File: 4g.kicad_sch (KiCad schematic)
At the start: 1 part, among them J6 Bus_M.2_Socket_B

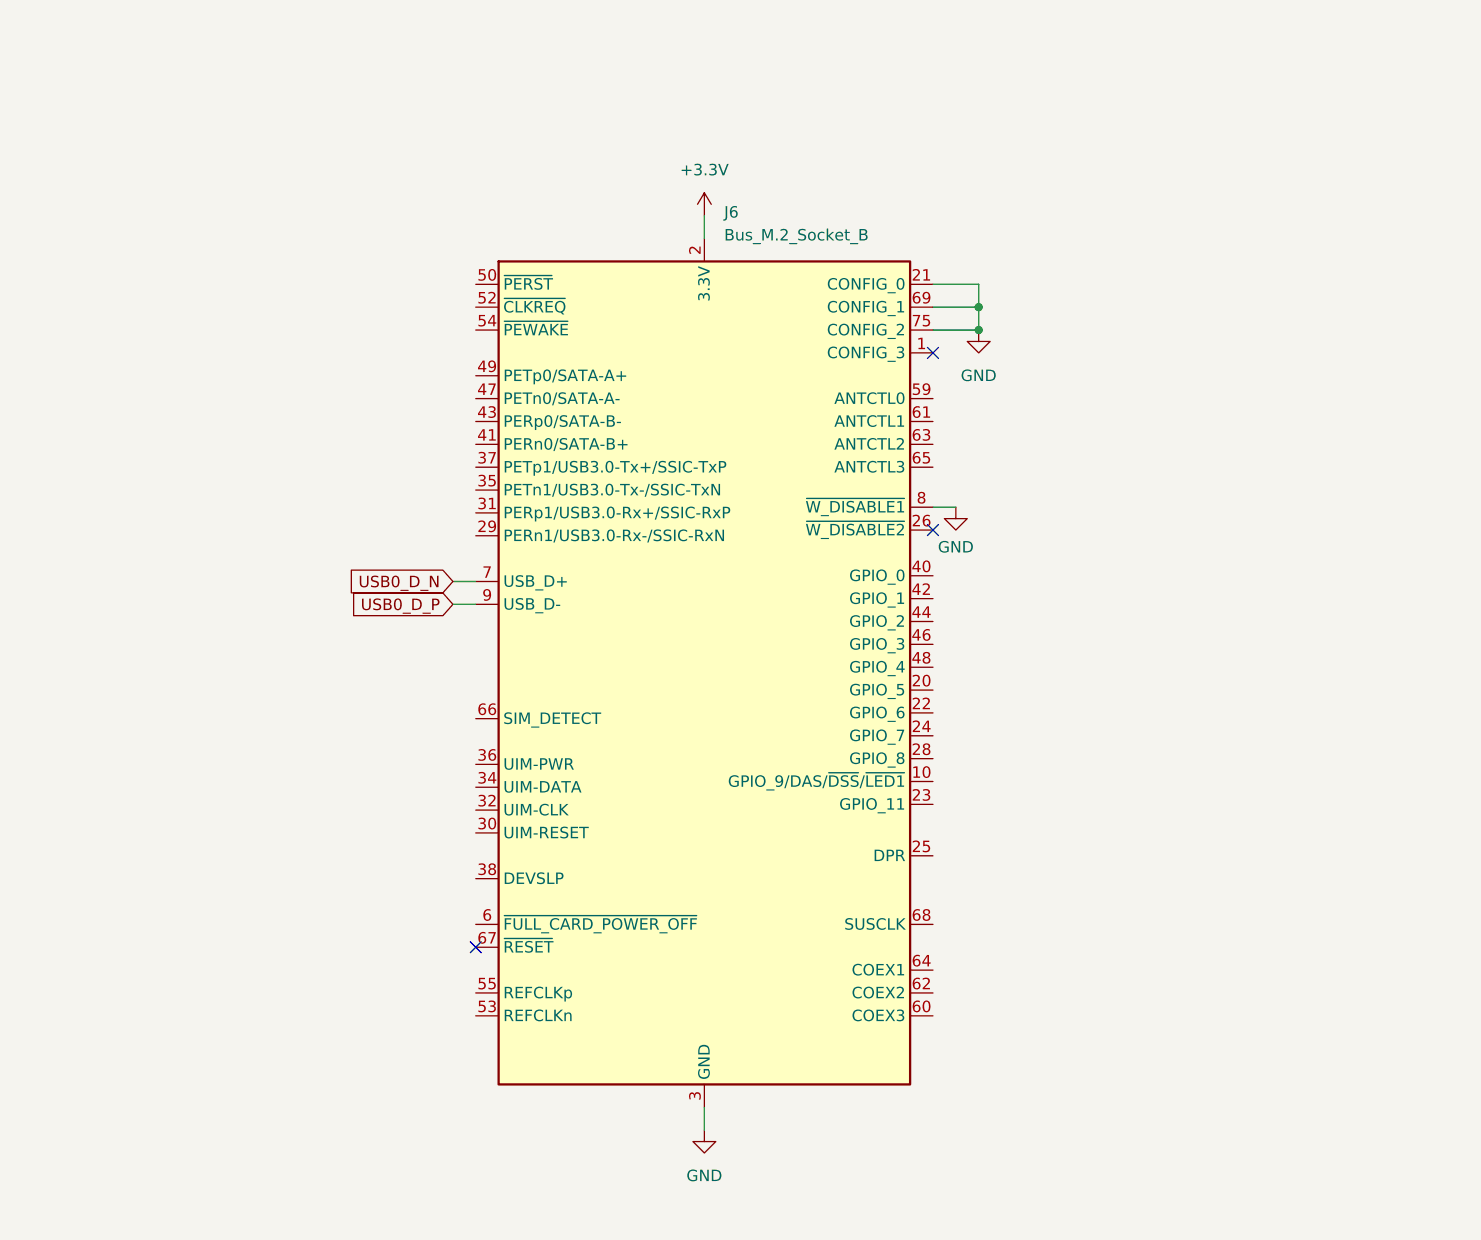
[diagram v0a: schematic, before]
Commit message: 4G V1 Done
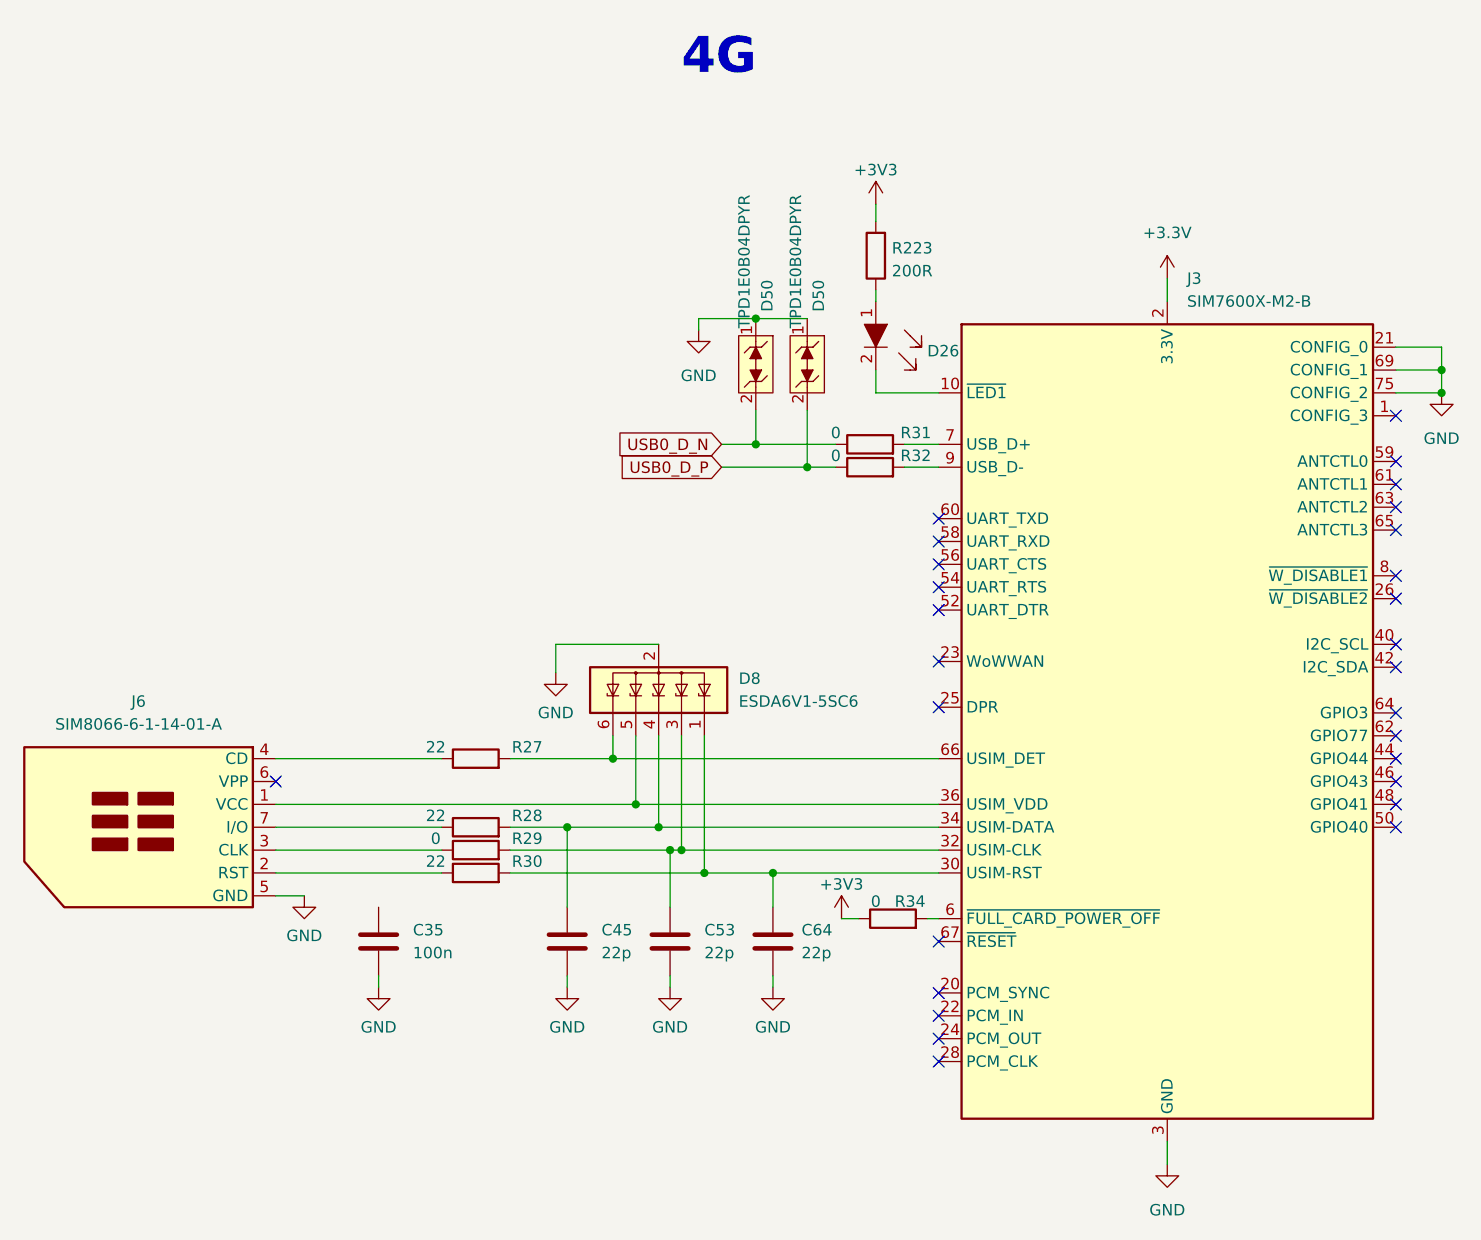
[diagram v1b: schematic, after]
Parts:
- removed J6: Bus_M.2_Socket_B, symbol Connector:Bus_M.2_Socket_B
- added C35: 100n, symbol Device:C
- added C45, C53, C64: 22p, symbol Device:C
- added D26: LTST-C190GKT, jetson-orin-baseboard-footprints:LED_0603, symbol jetson-orin-baseboard:LTST-C190GKT
- added D50 (x2): TPD1E0B04DPYR, jetson-orin-baseboard-footprints:XDFN-2_1x0.60mm, symbol jetson-orin-baseboard:TPD1E0B04DPYR
- added D8: ESDA6V1-5SC6, Package_TO_SOT_SMD:SOT-23-6, symbol Power_Protection:ESDA6V1-5SC6
- added J3: SIM7600X-M2-B, symbol jetson-orin-baseboard:SIM7600X-M2-B
- added J6: SIM8066-6-1-14-01-A, symbol jetson-orin-baseboard:SIM_Card_With_Detect
- added R223: R_200R_0402, jetson-orin-baseboard-footprints:0402-res, symbol jetson-orin-baseboard:R_200R_0402
- added R27, R28, R30: 22, symbol Device:R
- added R29, R31, R32, R34: 0, symbol Device:R
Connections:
- net +3.3V: now also J3.2 (3.3V), J3.4 (3.3V), J3.70 (3.3V), J3.72 (3.3V), J3.74 (3.3V)
- net GND: now also C35.2, C45.2, C53.2, C64.2, D50.1, D50.1, D8.2 (GND), J3.11 (GND), J3.21 (CONFIG_0), J3.27 (GND), J3.3 (GND), J3.33 (GND), J3.39 (GND), J3.45 (GND), J3.5 (GND), J3.51 (GND), J3.57 (GND), J3.69 (CONFIG_1), J3.71 (GND), J3.73 (GND), J3.75 (CONFIG_2), J6.5 (GND)
- net USB0_D_N: now also D50.2, R31.1
- net USB0_D_P: now also D50.2, R32.1
- new net: D26.2, J3.10 (~{LED1})
- new net: C64.1, D8.1 (IO1), J3.30 (USIM-RST), R30.2
- new net: C53.1, D8.3 (IO2), J3.32 (USIM-CLK), R29.2
- new net: C45.1, D8.4 (IO3), J3.34 (USIM-DATA), R28.2
- new net: D8.5 (IO4), J3.36 (USIM_VDD), J6.1 (VCC)
- new net: J3.6 (~{FULL_CARD_POWER_OFF}), R34.2
- new net: D8.6 (IO5), J3.66 (USIM_DET), R27.2
- new net: J3.7 (USB_D+), R31.2
- new net: J3.9 (USB_D-), R32.2
- new net: J6.7 (I/O), R28.1
- new net: D26.1, R223.1
- new net: J6.3 (CLK), R29.1
- new net: J6.4 (CD), R27.1
- new net: J6.2 (RST), R30.1
- new net +3V3: R223.2, R34.1
- no-connect marks 3 -> 28
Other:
- note added: "4G"
